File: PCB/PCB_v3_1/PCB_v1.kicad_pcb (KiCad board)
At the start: 4 copper layers, 100 x 35 mm, 62 parts, among them J1 LiPo Connection, J3 Altimax Power, J7 Conn_01x24_Male, J8 Conn_01x24_Male, J9 Thermocouples, SW1 SW_Push, SW2 SW_Push, U10 AIS1120SXTR, U11 RSCMRNE015PASE3, U12 RSCDJNI060PASE3, U2 TSR_1-2450, U4 Teensy3.5, U5 MAX31855KASA, U6 MAX31855KASA, U7 MAX31855KASA, U8 MAX31855KASA, U9 ADIS16470

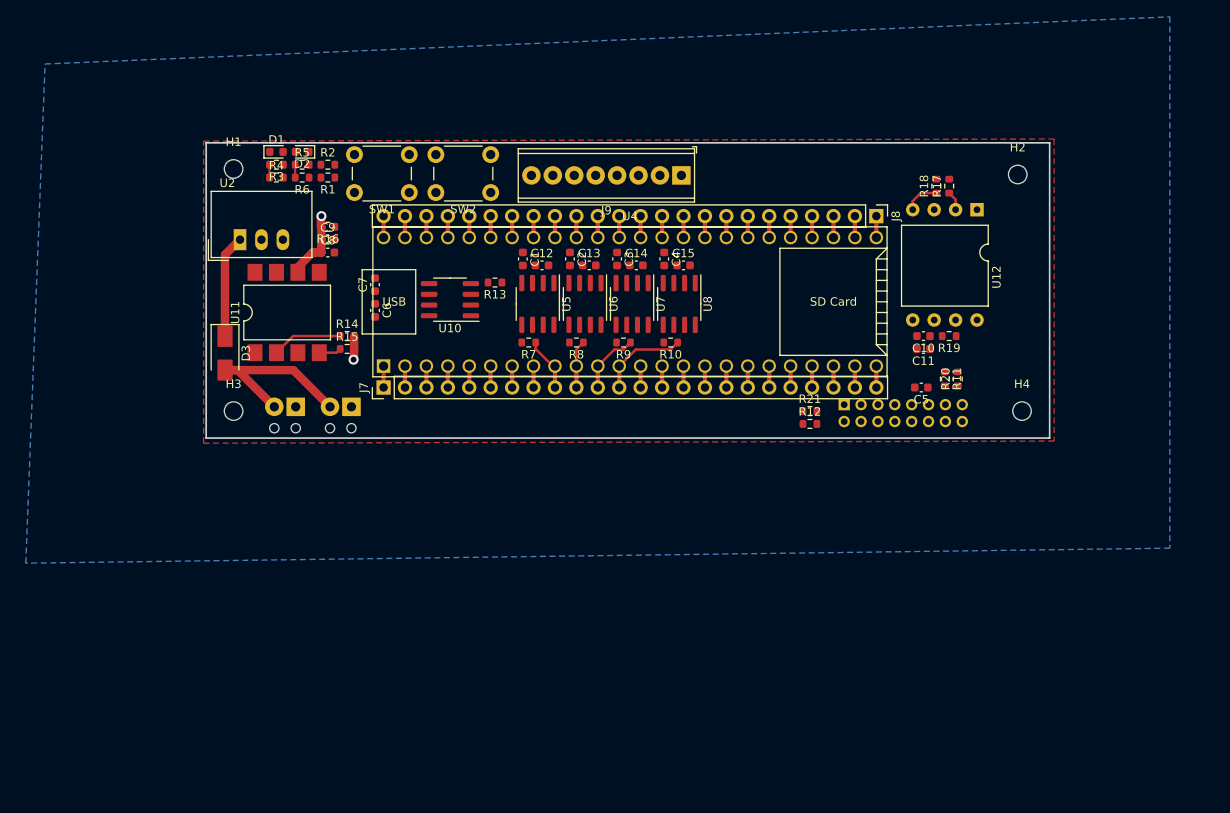
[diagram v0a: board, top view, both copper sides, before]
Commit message: Debug + update PCB
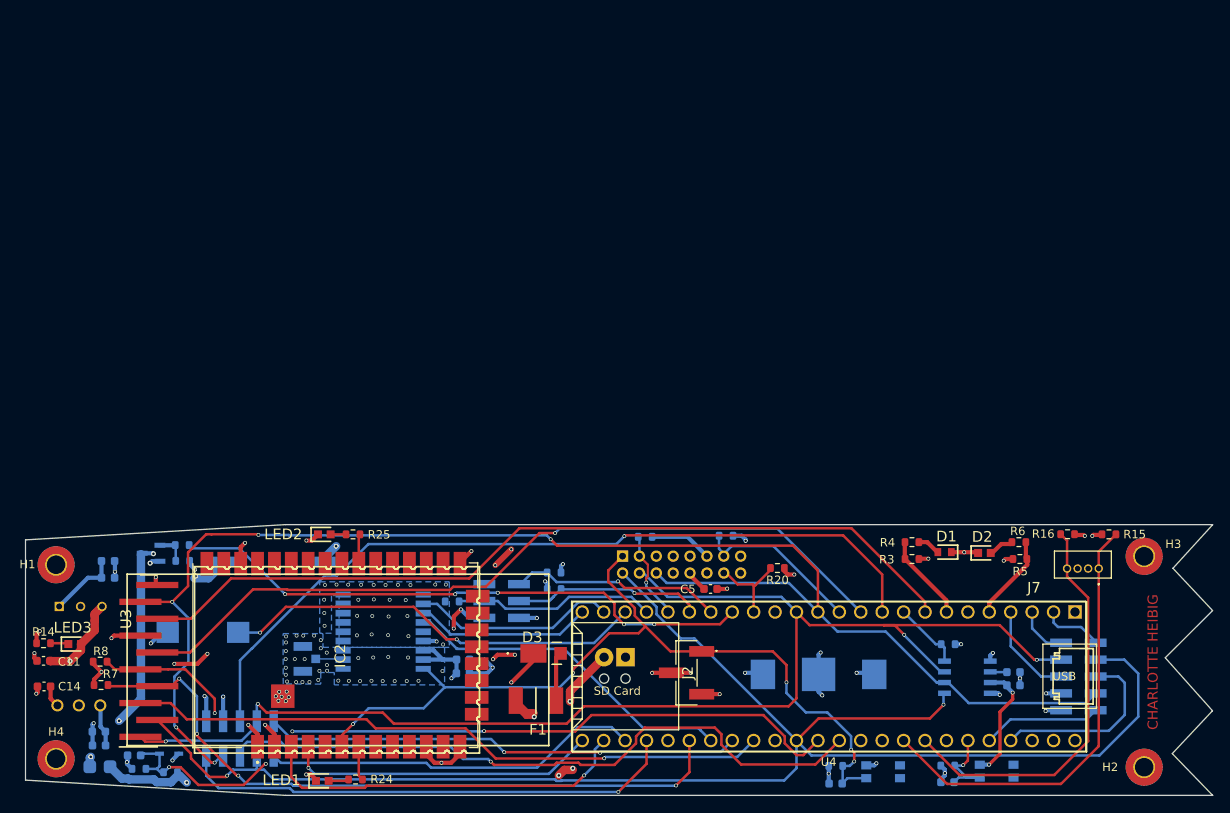
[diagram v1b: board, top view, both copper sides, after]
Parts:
- removed C15: 10nF, Capacitor_SMD:C_0603_1608Metric
- removed J8: Conn_01x24_Male, Connector_PinHeader_2.54mm:PinHeader_1x24_P2.54mm_Vertical
- removed J9: Thermocouples, TerminalBlock_Phoenix:TerminalBlock_Phoenix_MPT-0,5-8-2.54_1x08_P2.54mm_Horizontal
- removed R17, R19, R21: 10kΩ, Resistor_SMD:R_0603_1608Metric
- removed the REF** at (173.1, 83.8)
- removed the REF** at (166.8, 82.8)
- removed SW1, SW2: SW_Push, Button_Switch_THT:SW_PUSH_6mm
- removed U11: RSCMRNE015PASE3, Package_DIP:SMDIP-8_W9.53mm
- removed U12: RSCDJNI060PASE3, CustomLib:DIP-8_W13.08mm
- removed U8: MAX31855KASA, Package_SO:SOIC-8_3.9x4.9mm_P1.27mm
- added D7: BZX584C3V3-G3-08, Library:SOD2513X110N, B.Cu at (95.6, 154.9)
- added F1: MINIASMDC150F_12-2, Library:MINISMDC050F2, F.Cu at (139.1, 148.6)
- added G***: LOGO, CustomLib:flamme, B.Cu at (124.0, 151.4)
- added G***: LOGO, CustomLib:lion, B.Cu at (135.7, 151.1)
- added IC1: MAX-7C-0, Library:MAX7C0, B.Cu at (121.0, 140.5)
- added IC2: XB8X-DMUS-001, Library:XBP9XDMRS001, F.Cu at (116.0, 143.5)
- added IC4: TSR_0.5-2433, Library:TSR-0.5-2433, B.Cu at (90.7, 151.2)
- added J2: 0878980304, Library:0878980304, F.Cu at (156.9, 145.3)
- added J4: CONUFL001-SMD-T, Library:CONUFL001-SMD, B.Cu at (111.5, 143.7)
- added J5: 57202G5203LF, Library:57202G5203LF, B.Cu at (135.0, 137.8)
- added L3: SMI-1027-T-5V-R, Library:SMI1027T5VR, B.Cu at (99.6, 140.5)
- added LED1: 150060GS75000, Library:LEDC1608X80N, F.Cu at (113.8, 158.1)
- added LED2: 150060GS75000, Library:LEDC1608X80N, F.Cu at (114.0, 128.9)
- added LED3: 150060GS75000, Library:LEDC1608X80N, F.Cu at (84.4, 141.9)
- added M1: MNMOS, Library:SOT95P237X112-3N, B.Cu at (93.5, 131.2)
- added R22: ?, Resistor_SMD:R_0603_1608Metric, B.Cu at (95.8, 157.1)
- added R23: ?, Resistor_SMD:R_0603_1608Metric, B.Cu at (92.0, 156.7)
- added R24: 24, Resistor_SMD:R_0603_1608Metric, F.Cu at (117.7, 158.0)
- added R25: 24, Resistor_SMD:R_0603_1608Metric, F.Cu at (117.4, 128.9)
- added R26: R, Resistor_SMD:R_0603_1608Metric, B.Cu at (97.2, 130.2)
- added R27: 10kOhm, Resistor_SMD:R_0603_1608Metric, B.Cu at (97.2, 132.1)
- added REF**: Charlotte, CustomLib:Charlotte, F.Cu at (212.2, 144.1)
- added SW3: MISM7R610, Library:MISM7R610, B.Cu at (108.2, 132.1)
- added U1: 57202G5205LF, Library:57202G5205LF, B.Cu at (203.4, 146.8)
- added U3: 1-2842102-0, Library:HUSRSP10W50P200_2000X200X550P, F.Cu at (93.2, 143.9)
- added VR1: TSR1-2450, Library:CONV_TSR1-2450, B.Cu at (85.1, 137.5)
- C1, C10, C2, C3, C6, C7, C9, R1, R11, R12, R13: moved to B.Cu
- C11: value 10uF -> 100nF
- C12: value 10nF -> 10uF; moved to B.Cu
- C13: value 10nF -> 100nF; moved to B.Cu
- C14: value 10nF -> 100nF
- C4: value 100nF -> 10uF; moved to B.Cu
- C8: value 100nF -> 1uF; moved to B.Cu
- D1: footprint LED_SMD:LED_0603_1608Metric -> Library:LEDC1608X45N
- D2: footprint LED_SMD:LED_0603_1608Metric -> Library:LEDC1608X80N
- D3: footprint Diode_SMD:D_SMA -> Library:V8PAN50M3I
- H1, H2, H3, H4: footprint MountingHole:MountingHole_2.2mm_M2 -> MountingHole:MountingHole_2.2mm_M2_Pad_TopBottom
- J1: value LiPo Connection -> Altimax Power
- J3: value Altimax Power -> LiPo Connection; footprint TerminalBlock_Phoenix:TerminalBlock_Phoenix_MPT-0,5-2-2.54_1x02_P2.54mm_Horizontal -> Library:pad2
- J7: value Conn_01x24_Male -> 1734598-4; footprint Connector_PinHeader_2.54mm:PinHeader_1x24_P2.54mm_Vertical -> Library:17345984
- R10, R18, R2, R9: value 10kΩ -> 10k; moved to B.Cu
- R14: value 10kΩ -> 10K
- R15, R16: value 10kΩ -> 10k
- R3: value 30Ω -> 100Ω
- R5: value 100Ω -> 24Ω
- R7, R8: value 10kΩ -> 10kOhm
- U10: footprint Package_SO:SOIC-8_3.9x4.9mm_P1.27mm -> Library:SOIC127P600X175-8N; moved to B.Cu
- U2: value TSR_1-2450 -> 57202G5205LF; footprint Converter_DCDC:Converter_DCDC_TRACO_TSR-1_THT -> Library:57202G5205LF; moved to B.Cu
- U5: value MAX31855KASA -> 3030; footprint Package_SO:SOIC-8_3.9x4.9mm_P1.27mm -> Library:3030; moved to B.Cu
- U6, U7: value MAX31855KASA -> switch; footprint Package_SO:SOIC-8_3.9x4.9mm_P1.27mm -> Library:RKC2SJF170SMTRLFS; moved to B.Cu
- U9: footprint Connector_PinHeader_2.00mm:PinHeader_2x08_P2.00mm_Vertical -> Library:PinHeader_2x08_P2.00mm_Vertical
- moved H4 121.7 mm to (82.2, 155.5)
- moved C11 110.7 mm to (80.7, 143.9)
- moved H3 109.3 mm to (211.2, 131.5)
- moved R1 101.3 mm to (187.9, 156.3)
- moved C10 100.8 mm to (88.4, 134.1), turned to 0 degrees
- moved R6 96.4 mm to (196.5, 131.8), turned to 0 degrees
- moved R5 96.0 mm to (196.4, 129.8), turned to 180 degrees
- moved R16 95.0 mm to (202.1, 128.9), turned to 0 degrees
- moved D2 93.8 mm to (192.3, 131.1), turned to 0 degrees
- moved R15 93.0 mm to (207.0, 128.9), turned to 180 degrees
- moved D1 92.3 mm to (187.5, 131.0), turned to 180 degrees
- moved C7 89.4 mm to (195.7, 146.8), turned to 0 degrees
- moved R4 87.9 mm to (183.7, 131.8)
- moved R3 87.6 mm to (183.7, 129.8)
- moved J7 87.5 mm to (205.8, 133.0), turned to 0 degrees
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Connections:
- C1 pad 1: GND -> /button1
- C1 pad 2: +3V3 -> GND
- C10 pad 1: +3V3 -> Net-(C10-Pad1)
- C11 pad 1: +3V3 -> +5V
- C12 pad 1: Net-(C12-Pad1) -> +5V
- C12 pad 2: Net-(C12-Pad2) -> GND
- C13 pad 1: Net-(C13-Pad1) -> +5V
- C13 pad 2: Net-(C13-Pad2) -> GND
- C14 pad 1: Net-(C14-Pad1) -> +3V3
- C14 pad 2: Net-(C14-Pad2) -> GND
- C2 pad 1: GND -> +3V3
- C2 pad 2: +3V3 -> /nReset
- C3 pad 1: GND -> +3V3
- C3 pad 2: +3V3 -> GND
- C4 pad 1: GND -> +3V3
- C4 pad 2: +3V3 -> GND
- C8 pad 1: +3V3 -> GND
- C8 pad 2: GND -> /bat_voltage
- C9 pad 1: +3V3 -> Net-(C10-Pad1)
- D3 pad 1: Net-(D3-Pad1) -> Net-(C10-Pad1)
- J1 pad 1: GND -> Net-(J1-Pad1)
- J1 pad 2: Net-(D3-Pad2) -> Net-(F1-Pad1)
- J3 pad 1: GND -> Net-(J1-Pad1)
- J3 pad 2: Net-(D3-Pad2) -> Net-(F1-Pad1)
- J7 pad 1: GND -> /load_minus
- J7 pad 2: Net-(J7-Pad2) -> GND
- J7 pad 3: Net-(J7-Pad3) -> +5V
- J7 pad 4: /INS/CS_AIS1120 -> /load_plus
- R1 pad 1: /I/O/Button1 -> /button1
- R10 pad 1: /Thermocouples/CS_TC4 -> GND
- R10 pad 2: +3V3 -> /aux2
- R11 pad 2: /INS/DR_ADIS16470 -> /dr_adis
- R12 pad 2: /INS/CS_ADIS16470 -> /cs_adis
- R13 pad 2: /INS/CS_AIS1120 -> /cs_acc
- R14 pad 1: /Pressure Sensors/DR_RSC015 -> Net-(LED3-Pad1)
- R14 pad 2: +3V3 -> GND
- R15 pad 1: /Pressure Sensors/CS_RSC015_ADC -> /load_minus
- R16 pad 1: /Pressure Sensors/CS_RSC015_EE -> /load_plus
- R18 pad 1: /Pressure Sensors/CS_RSC060_ADC -> +3V3
- R18 pad 2: +3V3 -> /nReset
- R2 pad 1: GND -> /aux3
- R2 pad 2: /I/O/Button2 -> GND
- R20 pad 1: /INS/SYNC_ADIS16470 -> GND
- R20 pad 2: GND -> /sync_adis
- R3 pad 2: /I/O/LED1 -> /led1
- R4 pad 1: /I/O/LED1 -> /led1
- R5 pad 1: /I/O/LED2 -> /led2
- R6 pad 2: /I/O/LED2 -> /led2
- R7 pad 1: /Thermocouples/CS_TC1 -> +3V3
- R7 pad 2: +3V3 -> /sda_i2c
- R8 pad 1: /Thermocouples/CS_TC2 -> +3V3
- R8 pad 2: +3V3 -> /scl_i2c
- R9 pad 1: /Thermocouples/CS_TC3 -> GND
- R9 pad 2: +3V3 -> /aux1
- U10 pad 4: /INS/CS_AIS1120 -> /cs_acc
- U2 pad 1: Net-(D3-Pad1) -> GND
- U2 pad 2: GND -> /cs_pressure_adc_2
- U2 pad 3: +5V -> +3V3
- U4 pad 10: /Thermocouples/CS_TC2 -> /cs_pressure_ee_2
- U4 pad 11: /Thermocouples/CS_TC3 -> /gp4_spi
- U4 pad 12: /Thermocouples/CS_TC4 -> /dr_adis
- U4 pad 15: +3V3 -> unconnected-(U4-Pad15)
- U4 pad 16: /INS/DR_ADIS16470 -> /sync_adis
- U4 pad 17: /INS/SYNC_ADIS16470 -> /enable_gnd
- U4 pad 18: /Pressure Sensors/DR_RSC060 -> /aux2
- U4 pad 19: /Pressure Sensors/CS_RSC060_ADC -> /aux1
- U4 pad 2: Net-(J7-Pad2) -> /cs_tc2
- U4 pad 20: /Pressure Sensors/CS_RSC060_EE -> /cs_adis
- U4 pad 21: Net-(J7-Pad21) -> /aux3
- U4 pad 22: Net-(J7-Pad22) -> /buzzer_input
- U4 pad 23: Net-(J7-Pad23) -> /tx_ublox
- U4 pad 24: Net-(J7-Pad24) -> /rx_ublox
- U4 pad 3: Net-(J7-Pad3) -> /cs_tc1
- U4 pad 30: Net-(J8-Pad1) -> /rx_xbee
- U4 pad 31: Net-(J8-Pad2) -> /tx_xbee
- U4 pad 32: /INS/RST_ADIS16470 -> /cs_tc4
- U4 pad 33: /INS/CS_ADIS16470 -> /cs_pressure_adc_2
- U4 pad 34: Net-(J8-Pad5) -> /scl_i2c
- U4 pad 35: Net-(J8-Pad6) -> /sda_i2c
- U4 pad 36: Net-(J8-Pad7) -> /timepulse_ublox
- U4 pad 37: Net-(J8-Pad8) -> /cs_tc3
- U4 pad 38: Net-(J8-Pad9) -> /gp0_spi
- U4 pad 39: Net-(J8-Pad10) -> GND
- U4 pad 4: /INS/CS_AIS1120 -> /cs_pressure_ee_1
- U4 pad 41: Net-(J8-Pad12) -> /bat_voltage
- U4 pad 42: /Pressure Sensors/DR_RSC015 -> /dr_pressure_2
- U4 pad 43: /Pressure Sensors/CS_RSC015_ADC -> unconnected-(U4-Pad43)
- U4 pad 44: /Pressure Sensors/CS_RSC015_EE -> unconnected-(U4-Pad44)
- U4 pad 45: Net-(J8-Pad16) -> /load_minus
- U4 pad 46: Net-(J8-Pad17) -> /load_plus
- U4 pad 47: /I/O/Button2 -> unconnected-(U4-Pad47)
- U4 pad 48: /I/O/Button1 -> /button1
- U4 pad 49: /I/O/LED2 -> /cs_pressure_adc_1
- U4 pad 5: Net-(J7-Pad5) -> /led2
- U4 pad 50: /I/O/LED1 -> /dr_pressure_1
- U4 pad 51: Net-(J8-Pad22) -> unconnected-(U4-Pad51)
- U4 pad 52: Net-(J8-Pad23) -> unconnected-(U4-Pad52)
- U4 pad 6: Net-(J7-Pad6) -> unconnected-(U4-Pad6)
- U4 pad 7: Net-(J7-Pad7) -> /led1
- U4 pad 8: Net-(J7-Pad8) -> /gp3_spi
- U4 pad 9: /Thermocouples/CS_TC1 -> /cs_acc
- U5 pad 1: GND -> /RTC_supply
- U5 pad 2: Net-(C12-Pad2) -> GND
- U5 pad 3: Net-(C12-Pad1) -> /RTC_supply
- U6 pad 1: GND -> /button1
- U6 pad 2: Net-(C13-Pad2) -> (no net)
- U6 pad 3: Net-(C13-Pad1) -> +3V3
- U6 pad 4: +3V3 -> (no net)
- U7 pad 1: GND -> /nReset
- U7 pad 2: Net-(C14-Pad2) -> (no net)
- U7 pad 3: Net-(C14-Pad1) -> GND
- U7 pad 4: +3V3 -> (no net)
- U9 pad 1: /INS/RST_ADIS16470 -> /nReset
- U9 pad 13: /INS/DR_ADIS16470 -> /dr_adis
- U9 pad 14: /INS/SYNC_ADIS16470 -> /sync_adis
- U9 pad 15: Net-(U9-Pad15) -> unconnected-(U9-Pad15)
- U9 pad 16: Net-(U9-Pad16) -> unconnected-(U9-Pad16)
- U9 pad 3: /INS/CS_ADIS16470 -> /cs_adis
- U9 pad 5: Net-(U9-Pad5) -> unconnected-(U9-Pad5)
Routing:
- net /SCK0: track 2.54 -> 189.7 mm, vias 0 -> 2
- net +5V: track 2.54 -> 177.3 mm, vias 0 -> 1
- net /MOSI0: track 2.54 -> 175.7 mm, vias 0 -> 5
- net /MISO0: track 2.54 -> 158.1 mm, vias 0 -> 4
- net Net-(J1-Pad1): track 0.00 -> 111.3 mm, vias 0 -> 4
- net /gp3_spi: track 0.00 -> 100.3 mm
- net /nReset: track 0.00 -> 98.9 mm, vias 0 -> 5
- net /cs_pressure_ee_2: track 0.00 -> 95.9 mm, vias 0 -> 1
- net Net-(F1-Pad1): track 0.00 -> 93.8 mm, vias 0 -> 5
- net /gp4_spi: track 0.00 -> 93.6 mm, vias 0 -> 1
- net /bat_voltage: track 0.00 -> 92.1 mm, vias 0 -> 4
- net /sda_i2c: track 0.00 -> 81.8 mm, vias 0 -> 4
- net /dr_pressure_2: track 0.00 -> 79.6 mm, vias 0 -> 1
- net /scl_i2c: track 0.00 -> 77.8 mm, vias 0 -> 1
- net /gp0_spi: track 0.00 -> 76.3 mm, vias 0 -> 1
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- added copper zone on In1.Cu, net +3V3
- added copper zone on In2.Cu, net GND
- removed copper zone on In2.Cu, net +3V3
- removed copper zone on F.Cu, net GND
- removed copper zone on In1.Cu, net GND
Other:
- board size 100 x 35 mm -> 140.8 x 32.1 mm
- net class Default removed
- board text added: "+"
- board text added: "-"
